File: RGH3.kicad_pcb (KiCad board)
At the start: 2 copper layers, 16 x 8.5 mm, 6 parts

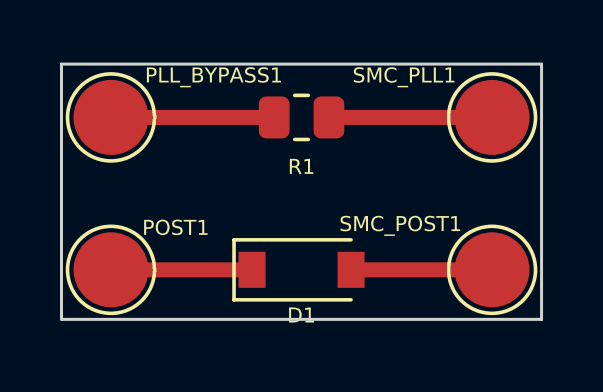
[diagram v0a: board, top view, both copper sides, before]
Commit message: Add files via upload
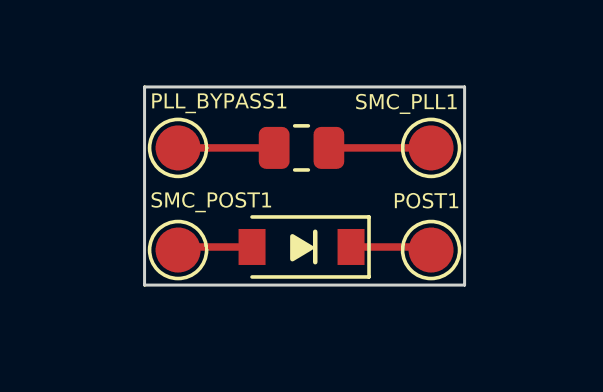
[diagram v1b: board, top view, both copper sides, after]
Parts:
- PLL_BYPASS1, POST1, SMC_PLL1, SMC_POST1: footprint TestPoint:TestPoint_Pad_D2.5mm -> TestPoint:TestPoint_Pad_D1.5mm
- moved POST1 10.7 mm to (146.6, 103.5)
- moved SMC_POST1 10.5 mm to (138.1, 103.5)
- moved PLL_BYPASS1 2.46 mm to (138.1, 100.1)
- moved SMC_PLL1 2.27 mm to (146.6, 100.1)
- moved R1 1.02 mm to (142.2, 100.1)
- moved D1 0.76 mm to (142.2, 103.4), turned to 180 degrees
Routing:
- net Net-(PLL_BYPASS1-Pad1): track 5.44 -> 3.20 mm
- net Net-(D1-Pad2): track 4.70 -> 2.51 mm
- net Net-(R1-Pad1): track 5.44 -> 3.41 mm
- net Net-(D1-Pad1): track 4.70 -> 2.71 mm
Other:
- board size 16 x 8.5 mm -> 10.7 x 6.6 mm
